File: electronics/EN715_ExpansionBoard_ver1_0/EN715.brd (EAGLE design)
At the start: 87 x 50 mm, 34 parts, among them IC1 FE1.1S

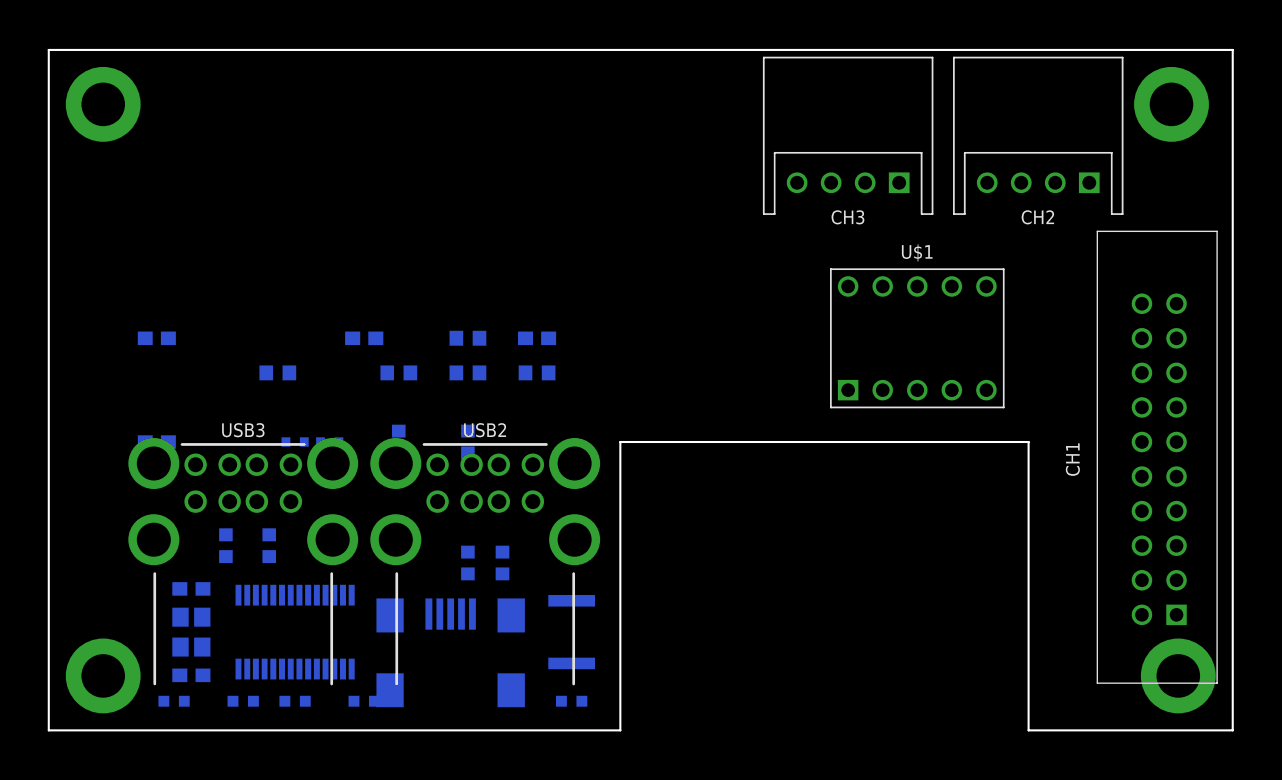
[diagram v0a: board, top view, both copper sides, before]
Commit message: Update Expansion board
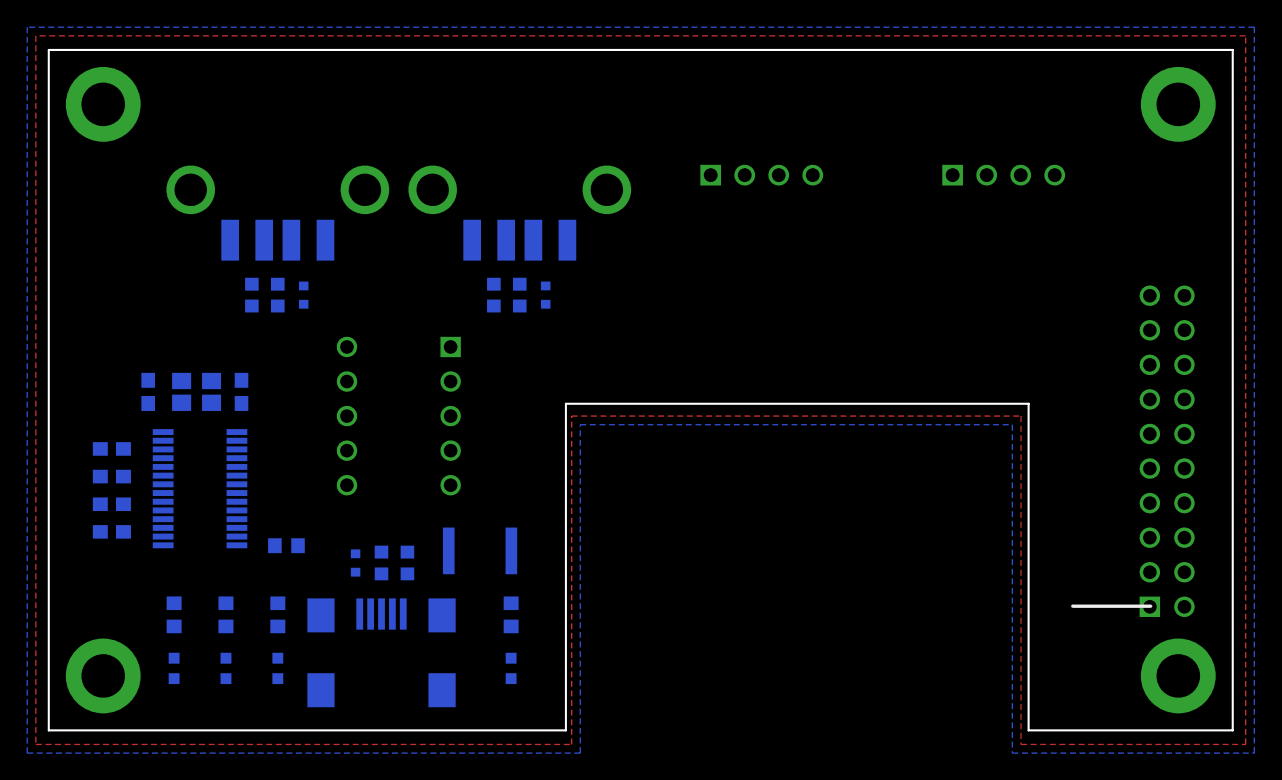
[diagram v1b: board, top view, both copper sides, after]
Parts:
- removed C11, C12, C13: 10u, rcl:C0603
- removed C14: 0.01u, rcl:C0603
- removed C15, C16: 22p, rcl:C0603
- removed D7: CG0603MLC-05E, CG0603MLC-05E:CG0603MLC-05E
- removed F6: MF-MSMF050, MF-MSMF:MF-MSMF050
- removed LED10, LED11, LED6, LED8, LED9: (no value), led:SML0603
- removed R15: 2.7k, rcl:R0603
- removed R19, R21, R22, R23: 1k, rcl:R0603
- removed U$1: MPU9250_MODULE, Strawberry-Linux_MPUP250_Module:MPU9250_MODULE
- added C1, C2, C3: 10u, rcl:C0603
- added C4: 0.01u, rcl:C0603
- added C5, C6: 22p, rcl:C0603
- added D1: CG0603MLC-05E, CG0603MLC-05E:CG0603MLC-05E
- added F1: MF-MSMF050, MF-MSMF:MF-MSMF050
- added FL3: BLM18SD220SN1D, BLM18SD220SN1D:BLM18SD220SN1D
- added LED1, LED2, LED3, LED4: (no value), led:SML0603
- added M1: MPU9250_MODULE, Strawberry-Linux_MPUP250_Module:MPU9250_MODULE
- added R1, R3, R4, R5: 1k, rcl:R0603
- added R2: 2.7k, rcl:R0603
- CH1: value HIF3FC-20PA-2.54DSA(71) -> 2X10; device HiroseConnector:HIF3FC-20PA-2.54DSA(71) -> Pin_socket:2X10
- USB1: value MINI_USB_5P_B_TYPE -> MINI_USB_B_SMD; device USB_Connector:MINI_USB_5P_B_TYPE -> USB_Connector:MINI_USB_B_SMD
- USB2, USB3: value USB_4P_A_TYPE_X2 -> USB_A_X1_SMD; device USB_Connector:USB_4P_A_TYPE_X2 -> USB_Connector:USB_A_X1_SMD
- moved USB2 46.7 mm to (-8.89, 25.0), flipped to the bottom, turned to 180 degrees
- moved USB3 46.7 mm to (-26.7, 25.0), flipped to the bottom, turned to 180 degrees
- moved D4 27.0 mm to (-10.8, 6.99)
- moved D6 27.0 mm to (-28.6, 6.99)
- moved FL2 19.2 mm to (-6.99, 6.99), turned to 90 degrees
- moved D5 18.4 mm to (-26.7, 6.99)
- moved CR1 17.7 mm to (-32.6, -0.13), turned to 0 degrees
- moved IC1 12.6 mm to (-32.4, -7.24), turned to 0 degrees
- moved D3 11.4 mm to (-8.89, 6.99)
- moved FL1 9.94 mm to (-21.0, -12.7), turned to 270 degrees
- moved D2 8.98 mm to (-19.1, -12.7), turned to 90 degrees
- moved CH3 6.37 mm to (8.89, 15.8), flipped to the bottom
- moved USB1 5.08 mm to (-19.1, -25.0)
- moved CH2 2.60 mm to (26.7, 15.8), flipped to the bottom
- moved CH1 0.83 mm to (38.7, -4.49), flipped to the bottom
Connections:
- removed net USB_A_SHIELD: D4.2, D5.2, D6.2, D7.2, FL1.1, USB2.MH1, USB2.MH2, USB2.MH3, USB2.MH4
- new net +3V3: CH1.2, CH2.2, CH3.2, M1.1, M1.2
- new net EN715_5V: CH1.1
- new net EN715_I2C1_SCL: CH1.8
- new net EN715_I2C1_SDA: CH1.6
- new net EN715_I2S0_LRCK_LS: CH1.20
- new net EN715_I2S0_SCLK_LS: CH1.14
- new net EN715_I2S0_SDIN_LS: CH1.18
- new net EN715_I2S0_SDOUT_LS: CH1.16
- new net EN715_ID_I2C_SCL: CH1.12
- new net EN715_ID_I2C_SDA: CH1.10
- new net EN715_SPI1_CS0_LS: CH1.17, M1.6
- new net EN715_SPI1_CS1_LS: CH1.19
- new net EN715_SPI1_MISO_LS: CH1.13, M1.5
- new net EN715_SPI1_MOSI_LS: CH1.15, M1.4
- new net EN715_SPI1_SCK_LS: CH1.11, M1.3
- new net EN715_UART2_RXD_3V3: CH1.7, CH3.4
- new net EN715_UART2_TXD_3V3: CH1.5, CH3.3
- new net N$1: CH2.3
- new net N$2: CH2.4
- new net USB_A_1_SHIELD: D3.2, D4.2, FL2.1, USB2.MH1, USB2.MH2
- new net USB_A_2_SHIELD: D5.2, D6.2, FL3.1, USB3.MH1, USB3.MH2
- net +5V: now also C3.1, C4.1, F1.1, R1.2, USB3.1; no longer C13.1, C14.1, F6.1, R19.2, USB2.5
- net AGND: now also C1.2, C2.2, C3.2, C4.2, C5.2, C6.2, CH1.3, CH1.4, CH1.9, CH2.1, CH3.1, FL3.2, LED1.C, M1.10, R2.1, R5.1, USB3.4; no longer C11.2, C12.2, C13.2, C14.2, C15.2, C16.2, LED6.C, R15.1, R23.1, USB2.8
- net B_FUSE_USB_MINI_B: now also F1.2; no longer F6.2
- net FE1.1S_DRV: now also LED2.A, LED3.A, LED4.A; no longer LED10.C, LED11.A, LED8.A, LED9.A
- net FE1.1S_DRV_LED_A: now also LED4.C, R5.2; no longer LED11.C, R23.2
- net FE1.1S_LED1_A: now also LED3.C, R4.2; no longer LED10.A, LED8.C, R21.2
- net FE1.1S_LED_1_B: now also R4.1; no longer R21.1
- net FE1.1S_LED_2_A: now also LED2.C, R3.2; no longer LED9.C, R22.2
- net FE1.1S_LED_2_B: now also R3.1; no longer R22.1
- net LED_USBIN: now also LED1.A, R1.1; no longer LED6.A, R19.1
- net REXT_FE1.1S: now also R2.2; no longer R15.2
- net USB-HUB_1_D+: now also D3.1, USB2.3
- net USB-HUB_1_D-: now also D4.1, USB2.2
- net USB-HUB_2_D+: now also D5.1, USB3.3; no longer D4.1, USB2.3
- net USB-HUB_2_D-: now also D6.1, USB3.2; no longer D5.1, USB2.2
- net USB-HUB_3_D+: no longer D6.1, USB2.7
- net USB-HUB_3_D-: no longer D7.1, USB2.6
- net USB_IN_D-: now also D1.1; no longer D3.1
- net USB_MINI_B_SHIELD: now also D1.2, FL1.1; no longer D3.2, FL2.1
- net VD18: now also C1.1; no longer C12.1
- net VD33: now also C2.1; no longer C11.1
- net XIN_FE1.1S: now also C5.1; no longer C15.1
- net XOUT_FE1.1S: now also C6.1; no longer C16.1
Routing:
- added copper zone on layer 1, net AGND
- added copper zone on layer 16, net AGND
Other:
- outline, holes or cut-outs redrawn
- board text added: "HUB Active"
- board text added: "Port1"
- board text added: "Port2"
- board text added: "USB Input state"
- board text added: "^UART"
- board text added: "^USB Port 1"
- board text added: "^USB Port 2"
